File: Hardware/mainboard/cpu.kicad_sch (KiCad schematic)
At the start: 26 parts, among them SW102 DNP, U100 MCIMX6Y2DVM09AB, Y101 24MHz, Y102 32.768kHz

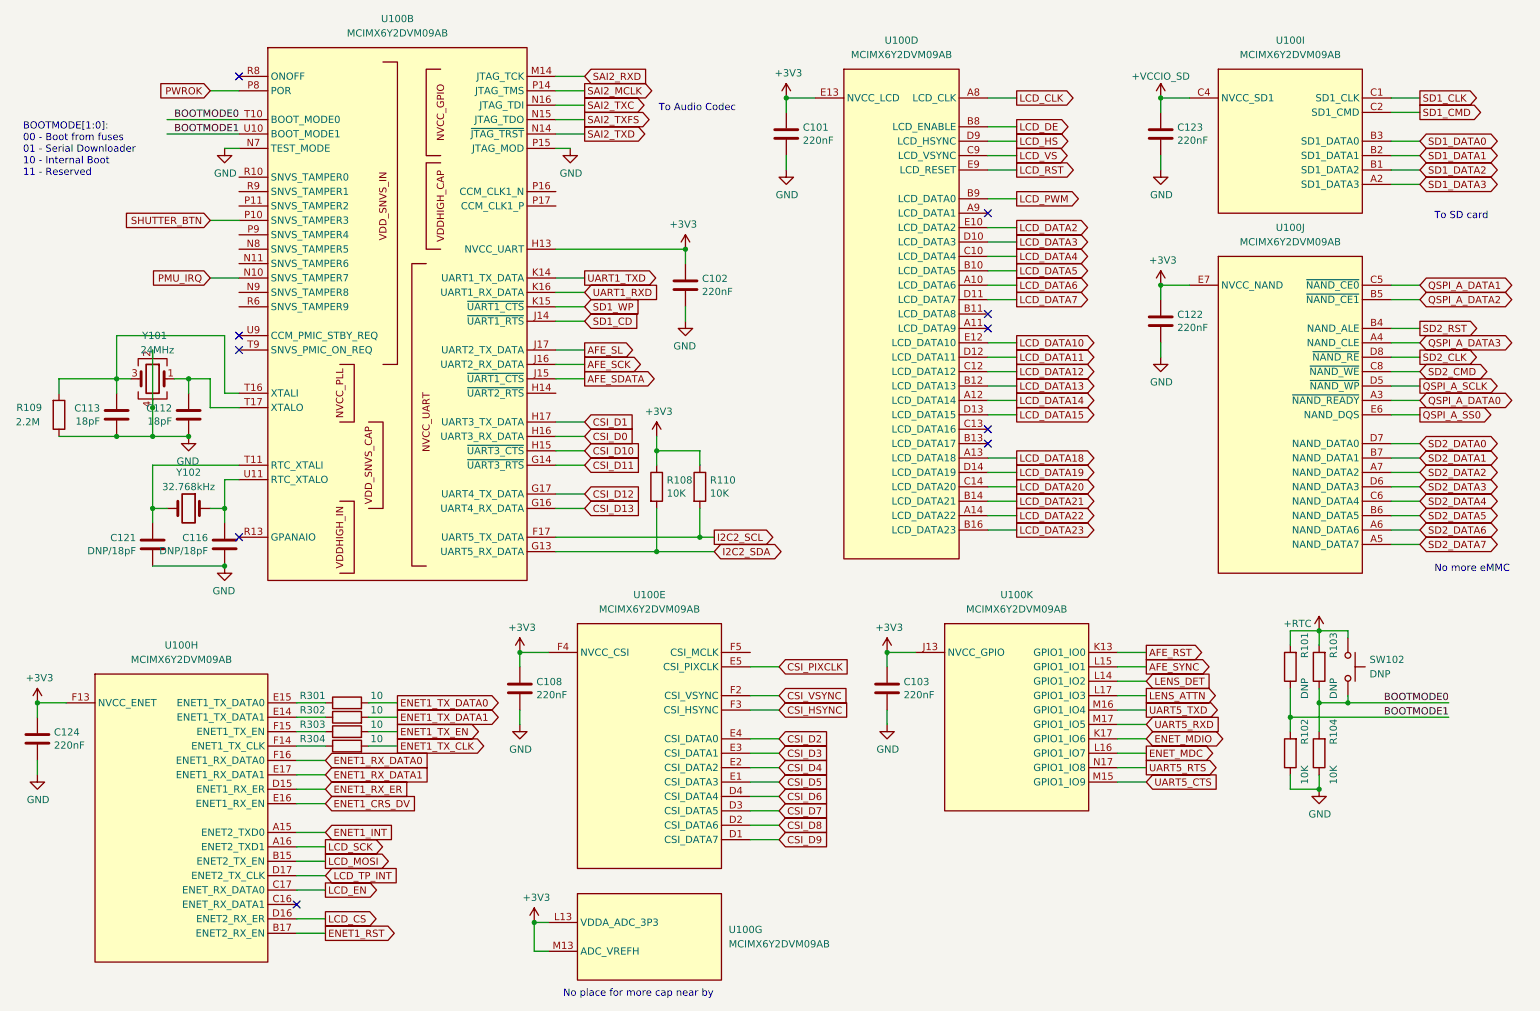
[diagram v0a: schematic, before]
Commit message: New PCB rev
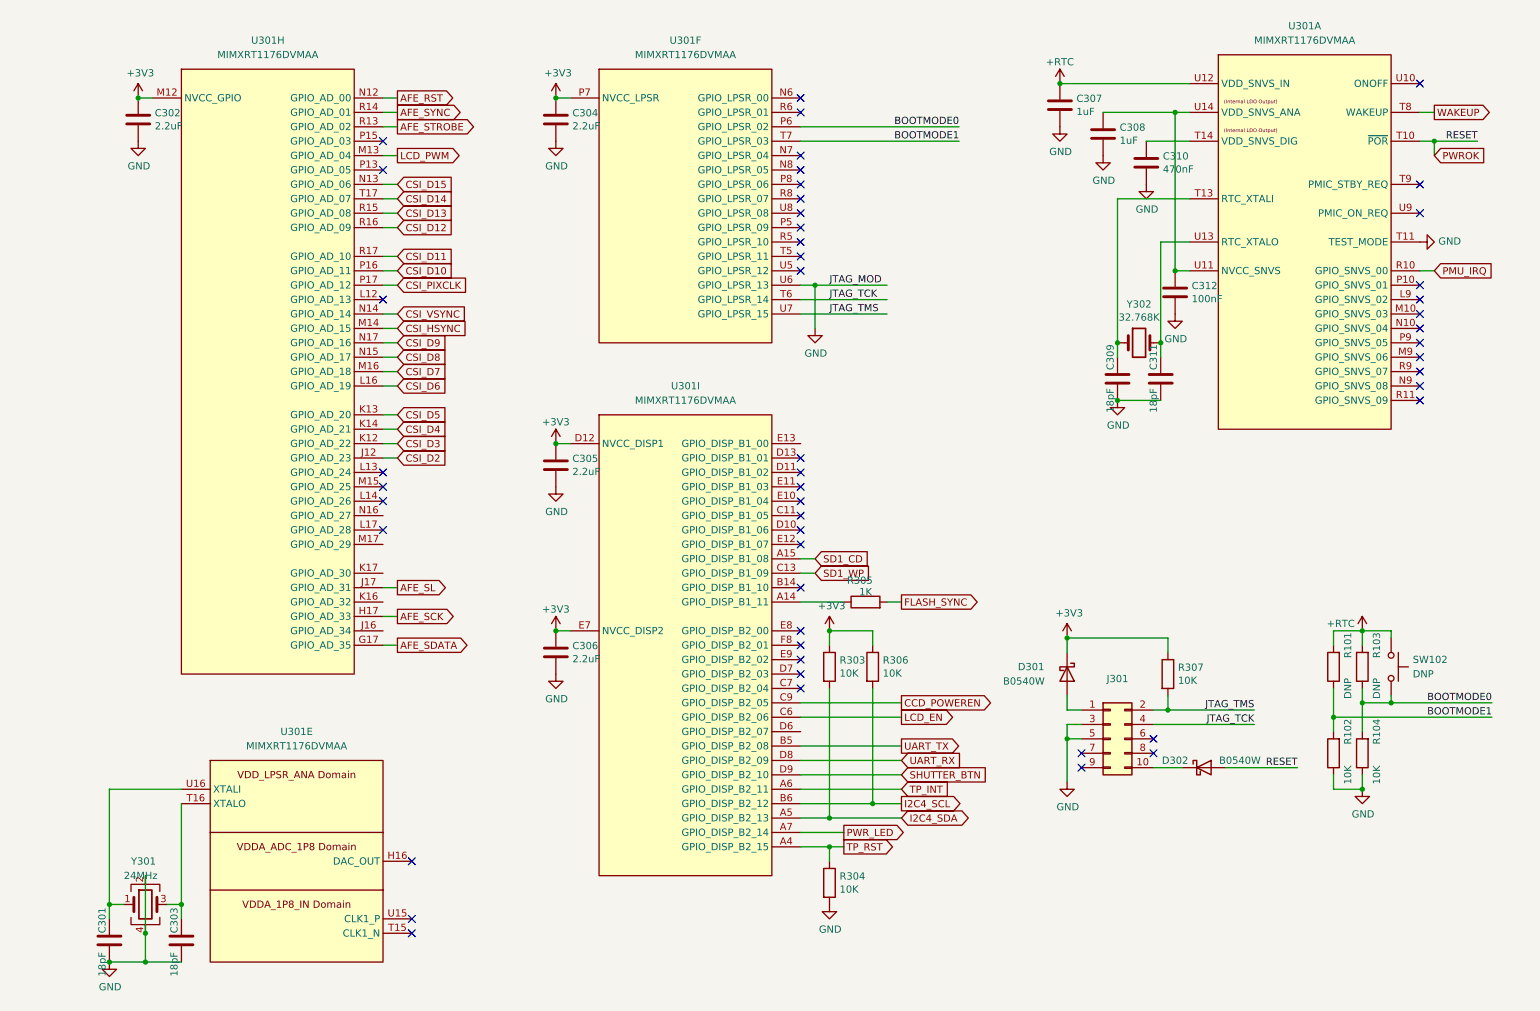
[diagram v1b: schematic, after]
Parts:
- removed C101, C102, C103, C108, C122, C123, C124: 220nF, Capacitor_SMD:C_0402_1005Metric, symbol Device:C
- removed C112, C113: 18pF, Capacitor_SMD:C_0402_1005Metric, symbol Device:C
- removed C116, C121: DNP/18pF, Capacitor_SMD:C_0402_1005Metric, symbol Device:C
- removed R108, R110: 10K, Resistor_SMD:R_0402_1005Metric, symbol Device:R
- removed R109: 2.2M, Resistor_SMD:R_0402_1005Metric, symbol Device:R
- removed R301, R302: 10, Resistor_SMD:R_0402_1005Metric, symbol Device:R
- removed U100: MCIMX6Y2DVM09AB, footprints:BGA-289_17x17_14.0x14.0mm, symbol symbols:MCIMX6Y7DVM09AB
- removed Y101: 24MHz, Oscillator:Oscillator_SMD_Abracon_ASE-4Pin_3.2x2.5mm, symbol Device:Crystal_GND24
- removed Y102: 32.768kHz, Crystal:Crystal_SMD_TXC_9HT11-2Pin_2.0x1.2mm_HandSoldering, symbol Device:Crystal
- added C301, C303, C309, C311: 18pF, Capacitor_SMD:C_0402_1005Metric, symbol Device:C
- added C302, C304, C305, C306: 2.2uF, Capacitor_SMD:C_0402_1005Metric, symbol Device:C
- added C307, C308: 1uF, Capacitor_SMD:C_0402_1005Metric, symbol Device:C
- added C310: 470nF, Capacitor_SMD:C_0402_1005Metric, symbol Device:C
- added C312: 100nF, Capacitor_SMD:C_0402_1005Metric, symbol Device:C
- added D301, D302: B0540W, Diode_SMD:D_SOD-323, symbol Device:D_Schottky
- added J301: Conn_02x05_Odd_Even, Connector_PinHeader_1.27mm:PinHeader_2x05_P1.27mm_Vertical_SMD, symbol Connector_Generic:Conn_02x05_Odd_Even
- added R305: 1K, Resistor_SMD:R_0402_1005Metric, symbol Device:R
- added R306, R307: 10K, Resistor_SMD:R_0402_1005Metric, symbol Device:R
- added U301: MIMXRT1176DVMAA, footprints:BGA-289_17x17_14.0x14.0mm, symbol symbols:MIMXRT1176DVMAA
- added Y301: 24MHz, Oscillator:Oscillator_SMD_Abracon_ASE-4Pin_3.2x2.5mm, symbol Device:Crystal_GND24
- added Y302: 32.768K, Crystal:Crystal_SMD_TXC_9HT11-2Pin_2.0x1.2mm_HandSoldering, symbol Device:Crystal
- R303, R304: value 10 -> 10K
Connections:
- net ENET1_TX_CLK is gone; now on net GND: R304.2
- net +3V3: now also R303.1, C302.1, C304.1, C305.1, C306.1, D301.1 (K), R306.1, R307.1, U301.D12 (NVCC_DISP1), U301.E7 (NVCC_DISP2), U301.M12 (NVCC_GPIO), U301.P7 (NVCC_LPSR)
- net +RTC: now also C307.1, U301.U12 (VDD_SNVS_IN)
- net AFE_RST: now also U301.N12 (GPIO_AD_00)
- net AFE_SCK: now also U301.H17 (GPIO_AD_33)
- net AFE_SDATA: now also U301.G17 (GPIO_AD_35)
- net AFE_SL: now also U301.J17 (GPIO_AD_31)
- net AFE_SYNC: now also U301.R14 (GPIO_AD_01)
- net BOOTMODE0: now also U301.P6 (GPIO_LPSR_02)
- net BOOTMODE1: now also U301.T7 (GPIO_LPSR_03)
- net CSI_D10: now also U301.P16 (GPIO_AD_11)
- net CSI_D11: now also U301.R17 (GPIO_AD_10)
- net CSI_D12: now also U301.R16 (GPIO_AD_09)
- net CSI_D13: now also U301.R15 (GPIO_AD_08)
- net CSI_D2: now also U301.J12 (GPIO_AD_23)
- net CSI_D3: now also U301.K12 (GPIO_AD_22)
- net CSI_D4: now also U301.K14 (GPIO_AD_21)
- net CSI_D5: now also U301.K13 (GPIO_AD_20)
- net CSI_D6: now also U301.L16 (GPIO_AD_19)
- net CSI_D7: now also U301.M16 (GPIO_AD_18)
- net CSI_D8: now also U301.N15 (GPIO_AD_17)
- net CSI_D9: now also U301.N17 (GPIO_AD_16)
- net CSI_HSYNC: now also U301.M14 (GPIO_AD_15)
- net CSI_PIXCLK: now also U301.P17 (GPIO_AD_12)
- net CSI_VSYNC: now also U301.N14 (GPIO_AD_14)
- net GND: now also C301.2, C302.2, C303.2, C304.2, C305.2, C306.2, C307.2, C308.2, C309.1, C310.2, C311.1, C312.2, J301.3 (Pin_3), J301.5 (Pin_5), U301.T11 (TEST_MODE), U301.U6 (GPIO_LPSR_13), Y301.2, Y301.4
- net LCD_EN: now also U301.C6 (GPIO_DISP_B2_06)
- net LCD_PWM: now also U301.M13 (GPIO_AD_04)
- net PMU_IRQ: now also U301.R10 (GPIO_SNVS_00)
- net PWROK: now also D302.2 (A), U301.T10 (~{POR})
- net SD1_CD: now also U301.A15 (GPIO_DISP_B1_08)
- net SD1_WP: now also U301.C13 (GPIO_DISP_B1_09)
- net SHUTTER_BTN: now also U301.D9 (GPIO_DISP_B2_10)
- net TP_RST: now reaches R304.1
- net TP_RST: now also U301.A4 (GPIO_DISP_B2_15)
- net ENET1_TX_EN renamed I2C4_SDA
- net I2C4_SDA: now also U301.A5 (GPIO_DISP_B2_13)
- new net: R305.1, U301.A14 (GPIO_DISP_B1_11)
- new net: C301.1, U301.U16 (XTALI), Y301.1
- new net: D301.2 (A), J301.1 (Pin_1)
- new net: C303.1, U301.T16 (XTALO), Y301.3
- new net: C309.2, U301.T13 (RTC_XTALI), Y302.1
- new net: C310.1, U301.T14 (VDD_SNVS_DIG)
- new net: C308.1, C312.1, U301.U11 (NVCC_SNVS), U301.U14 (VDD_SNVS_ANA)
- new net: C311.2, U301.U13 (RTC_XTALO), Y302.2
- new net: D302.1 (K), J301.10 (Pin_10)
- new net AFE_STROBE: U301.R13 (GPIO_AD_02)
- new net CCD_POWEREN: U301.C9 (GPIO_DISP_B2_05)
- new net CSI_D14: U301.T17 (GPIO_AD_07)
- new net CSI_D15: U301.N13 (GPIO_AD_06)
- new net FLASH_SYNC: R305.2
- new net I2C4_SCL: R306.2, U301.B6 (GPIO_DISP_B2_12)
- new net JTAG_TCK: J301.4 (Pin_4), U301.T6 (GPIO_LPSR_14)
- new net JTAG_TMS: J301.2 (Pin_2), R307.2, U301.U7 (GPIO_LPSR_15)
- new net PWR_LED: U301.A7 (GPIO_DISP_B2_14)
- new net TP_INT: U301.A6 (GPIO_DISP_B2_11)
- new net UART_RX: U301.D8 (GPIO_DISP_B2_09)
- new net UART_TX: U301.B5 (GPIO_DISP_B2_08)
- new net WAKEUP: U301.T8 (WAKEUP)
- no-connect marks 10 -> 50
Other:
- note removed: "BOOTMODE[1:0]: 00 - Boot from fuses 01 - Serial Downloader 10 - Internal Boot 11 - Reserved"
- note removed: "No more eMMC"
- note removed: "No place for more cap near by"
- note removed: "To Audio Codec"
- note removed: "To SD card"
- moved on the sheet: R101, R102, R103, R104, SW102

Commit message: Update PCB files to rev 0.6 used for production
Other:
- company: Copyright 2022 Wenting Zhang -> Copyright 2023 Wenting Zhang
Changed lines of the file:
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@@
   (title_block
     (title "Sitina 1 Mainboard")
-    (date "2022-04-28")
-    (rev "R0.1")
-    (company "Copyright 2022 Wenting Zhang")
+    (date "2023-03-16")
+    (rev "R0.6")
+    (company "Copyright 2023 Wenting Zhang")
     (comment 2 "MERCHANTABILITY, SATISFACTORY QUALITY AND FITNESS FOR A PARTICULAR PURPOSE.")
     (comment 3 "This source is distributed WITHOUT ANY EXPRESS OR IMPLIED WARRANTY, INCLUDING OF")
